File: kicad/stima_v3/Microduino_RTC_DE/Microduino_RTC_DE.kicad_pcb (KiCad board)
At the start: 2 copper layers, 25.5 x 27.9 mm, 16 parts, among them P1 CONN_1x27, U1 PCF8563, Y1 32,762 kHz

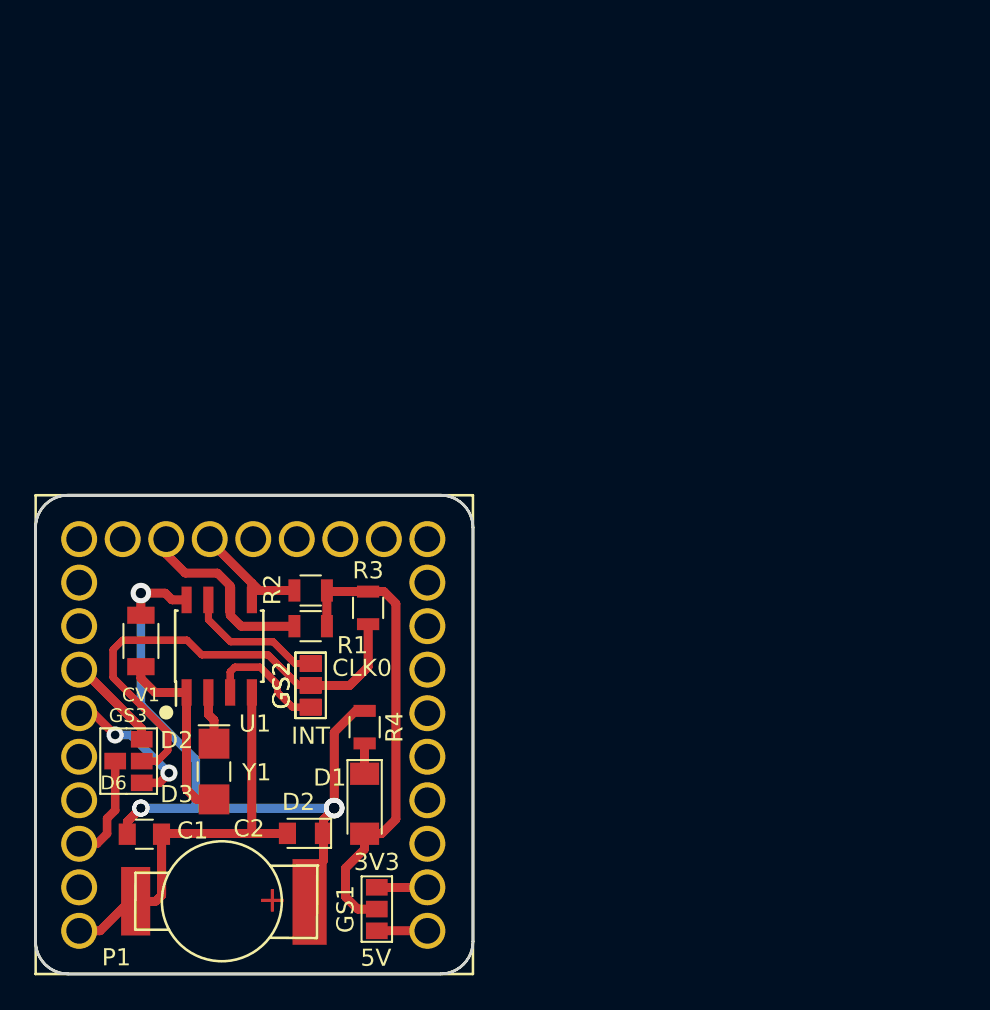
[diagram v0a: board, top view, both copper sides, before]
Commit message: reapload kicad scheme
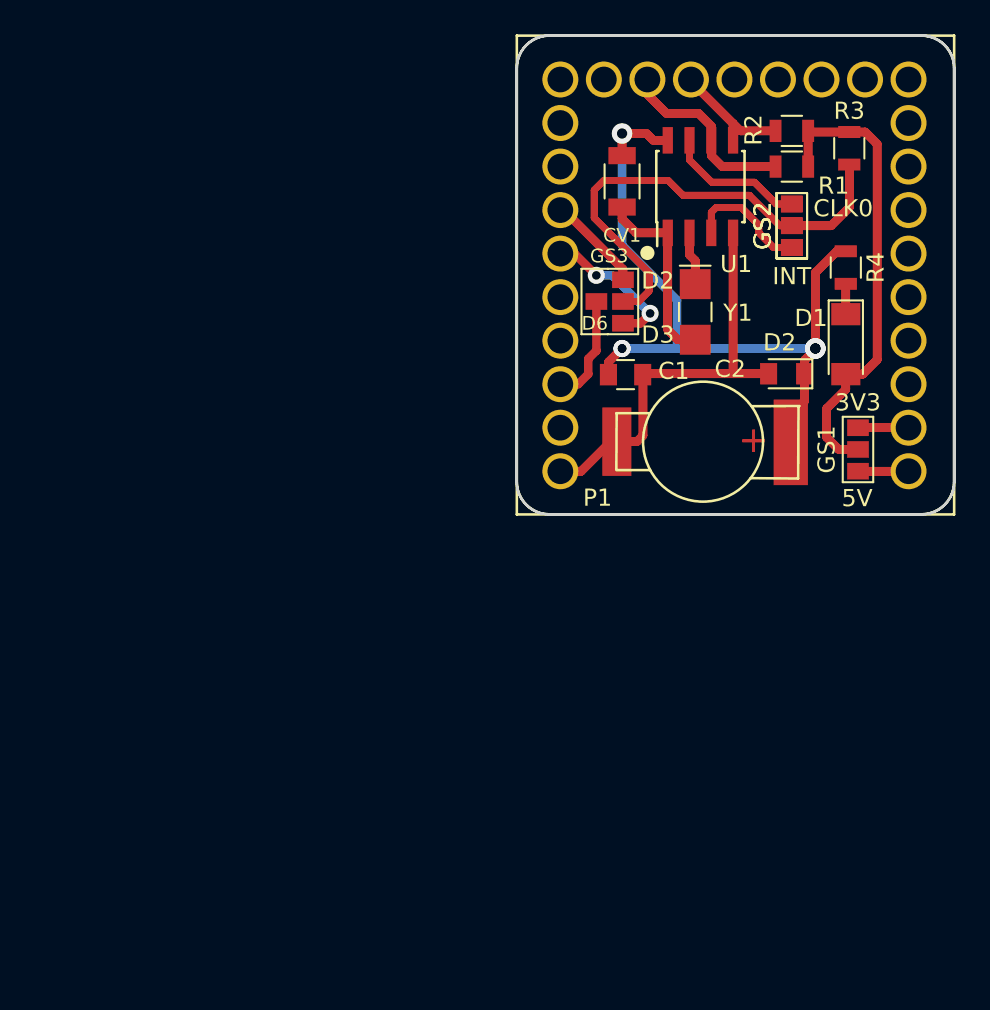
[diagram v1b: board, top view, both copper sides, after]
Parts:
- moved D1 38.8 mm to (157.9, 80.7)
- moved GS1 38.8 mm to (158.6, 86.9)
- moved R4 38.8 mm to (157.9, 76.3)
- moved GS2 38.8 mm to (154.7, 73.8) (x2)
- moved GS3 38.8 mm to (144.9, 78.3)
- moved P1 38.8 mm to (161.6, 88.2)
- moved R2 38.8 mm to (154.7, 68.3)
- moved C1 38.8 mm to (145.0, 82.5)
- moved C2 38.8 mm to (149.6, 86.4)
- moved CV1 38.8 mm to (144.8, 71.2)
- moved D2 38.8 mm to (154.4, 82.5)
- moved R1 38.8 mm to (154.7, 70.4)
- moved U1 38.8 mm to (149.4, 71.6)
- moved Y1 38.8 mm to (149.1, 78.9)
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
